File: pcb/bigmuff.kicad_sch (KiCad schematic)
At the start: 46 parts, among them Q1 BC549, Q2 BC549, Q3 BC549, Q4 BC549

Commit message: update pcb
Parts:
- C1, C6, C8: footprint Capacitor_THT:CP_Radial_Tantal_D4.5mm_P5.00mm -> Capacitor_THT:C_Axial_L5.1mm_D3.1mm_P7.50mm_Horizontal
- C10, C11, C12, C13, C2, C3, C4, C5, C7, C9: footprint Capacitor_THT:C_Disc_D4.3mm_W1.9mm_P5.00mm -> Capacitor_THT:C_Axial_L5.1mm_D3.1mm_P7.50mm_Horizontal
- R1, R10, R11, R12, R13, R14, R15, R16, R17, R18, R19, R2, R20, R21, R22, R3, R4, R5, R6, R7, R8, R9: footprint Resistor_THT:R_Axial_DIN0207_L6.3mm_D2.5mm_P7.62mm_Horizontal -> Resistor_THT:R_Axial_DIN0207_L6.3mm_D2.5mm_P10.16mm_Horizontal
- RV1, RV2, RV3: footprint Potentiometer_THT:Potentiometer_Alpha_RD901F-40-00D_Single_Vertical -> Potentiometer_THT:Potentiometer_Alps_RK09L_Single_Vertical
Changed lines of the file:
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@@
 			)
 		)
-		(property "Footprint" "Resistor_THT:R_Axial_DIN0207_L6.3mm_D2.5mm_P7.62mm_Horizontal"
+		(property "Footprint" "Resistor_THT:R_Axial_DIN0207_L6.3mm_D2.5mm_P10.16mm_Horizontal"
 			(at 34.29 66.802 90)
 			(effects
@@
 			)
 		)
-		(property "Footprint" "Resistor_THT:R_Axial_DIN0207_L6.3mm_D2.5mm_P7.62mm_Horizontal"
+		(property "Footprint" "Resistor_THT:R_Axial_DIN0207_L6.3mm_D2.5mm_P10.16mm_Horizontal"
 			(at 198.882 74.93 90)
 			(effects
@@
 			)
 		)
-		(property "Footprint" "Resistor_THT:R_Axial_DIN0207_L6.3mm_D2.5mm_P7.62mm_Horizontal"
+		(property "Footprint" "Resistor_THT:R_Axial_DIN0207_L6.3mm_D2.5mm_P10.16mm_Horizontal"
 			(at 53.34 165.608 90)
 			(effects
@@
 			)
 		)
-		(property "Footprint" "Resistor_THT:R_Axial_DIN0207_L6.3mm_D2.5mm_P7.62mm_Horizontal"
+		(property "Footprint" "Resistor_THT:R_Axial_DIN0207_L6.3mm_D2.5mm_P10.16mm_Horizontal"
 			(at 69.342 81.28 90)
 			(effects
@@
 			)
 		)
-		(property "Footprint" "Resistor_THT:R_Axial_DIN0207_L6.3mm_D2.5mm_P7.62mm_Horizontal"
+		(property "Footprint" "Resistor_THT:R_Axial_DIN0207_L6.3mm_D2.5mm_P10.16mm_Horizontal"
 			(at 198.882 49.53 90)
 			(effects
@@
 			)
 		)
-		(property "Footprint" "Resistor_THT:R_Axial_DIN0207_L6.3mm_D2.5mm_P7.62mm_Horizontal"
+		(property "Footprint" "Resistor_THT:R_Axial_DIN0207_L6.3mm_D2.5mm_P10.16mm_Horizontal"
 			(at 210.312 49.53 90)
 			(effects
@@
 			)
 		)
-		(property "Footprint" "Resistor_THT:R_Axial_DIN0207_L6.3mm_D2.5mm_P7.62mm_Horizontal"
+		(property "Footprint" "Resistor_THT:R_Axial_DIN0207_L6.3mm_D2.5mm_P10.16mm_Horizontal"
 			(at 73.66 157.988 90)
 			(effects
@@
 			)
 		)
-		(property "Footprint" "Potentiometer_THT:Potentiometer_Alpha_RD901F-40-00D_Single_Vertical"
+		(property "Footprint" "Potentiometer_THT:Potentiometer_Alps_RK09L_Single_Vertical"
 			(at 146.05 63.5 0)
 			(effects
@@
 			)
 		)
-		(property "Footprint" "Capacitor_THT:C_Disc_D4.3mm_W1.9mm_P5.00mm"
+		(property "Footprint" "Capacitor_THT:C_Axial_L5.1mm_D3.1mm_P7.50mm_Horizontal"
 			(at 82.55 57.4548 0)
 			(effects
@@
 			)
 		)
-		(property "Footprint" "Capacitor_THT:C_Disc_D4.3mm_W1.9mm_P5.00mm"
+		(property "Footprint" "Capacitor_THT:C_Axial_L5.1mm_D3.1mm_P7.50mm_Horizontal"
 			(at 66.04 44.7548 0)
 			(effects
@@
 			)
 		)
-		(property "Footprint" "Potentiometer_THT:Potentiometer_Alpha_RD901F-40-00D_Single_Vertical"
+		(property "Footprint" "Potentiometer_THT:Potentiometer_Alps_RK09L_Single_Vertical"
 			(at 85.09 68.58 0)
 			(effects
@@
 			)
 		)
-		(property "Footprint" "Capacitor_THT:C_Disc_D4.3mm_W1.9mm_P5.00mm"
+		(property "Footprint" "Capacitor_THT:C_Axial_L5.1mm_D3.1mm_P7.50mm_Horizontal"
 			(at 46.99 162.8648 0)
 			(effects
@@
 			)
 		)
-		(property "Footprint" "Potentiometer_THT:Potentiometer_Alpha_RD901F-40-00D_Single_Vertical"
+		(property "Footprint" "Potentiometer_THT:Potentiometer_Alps_RK09L_Single_Vertical"
 			(at 232.41 66.04 0)
 			(effects
@@
 			)
 		)
-		(property "Footprint" "Resistor_THT:R_Axial_DIN0207_L6.3mm_D2.5mm_P7.62mm_Horizontal"
+		(property "Footprint" "Resistor_THT:R_Axial_DIN0207_L6.3mm_D2.5mm_P10.16mm_Horizontal"
 			(at 113.792 173.99 90)
 			(effects
@@
 			)
 		)
-		(property "Footprint" "Resistor_THT:R_Axial_DIN0207_L6.3mm_D2.5mm_P7.62mm_Horizontal"
+		(property "Footprint" "Resistor_THT:R_Axial_DIN0207_L6.3mm_D2.5mm_P10.16mm_Horizontal"
 			(at 109.22 165.608 90)
 			(effects
@@
 			)
 		)
-		(property "Footprint" "Capacitor_THT:C_Disc_D4.3mm_W1.9mm_P5.00mm"
+		(property "Footprint" "Capacitor_THT:C_Axial_L5.1mm_D3.1mm_P7.50mm_Horizontal"
 			(at 195.58 59.9948 0)
 			(effects
@@
 			)
 		)
-		(property "Footprint" "Resistor_THT:R_Axial_DIN0207_L6.3mm_D2.5mm_P7.62mm_Horizontal"
+		(property "Footprint" "Resistor_THT:R_Axial_DIN0207_L6.3mm_D2.5mm_P10.16mm_Horizontal"
 			(at 144.272 46.99 90)
 			(effects
@@
 			)
 		)
-		(property "Footprint" "Capacitor_THT:CP_Radial_Tantal_D4.5mm_P5.00mm"
+		(property "Footprint" "Capacitor_THT:C_Axial_L5.1mm_D3.1mm_P7.50mm_Horizontal"
 			(at 62.23 129.2352 0)
 			(effects
@@
 			)
 		)
-		(property "Footprint" "Resistor_THT:R_Axial_DIN0207_L6.3mm_D2.5mm_P7.62mm_Horizontal"
+		(property "Footprint" "Resistor_THT:R_Axial_DIN0207_L6.3mm_D2.5mm_P10.16mm_Horizontal"
 			(at 128.27 157.988 90)
 			(effects
@@
 			)
 		)
-		(property "Footprint" "Capacitor_THT:C_Disc_D4.3mm_W1.9mm_P5.00mm"
+		(property "Footprint" "Capacitor_THT:C_Axial_L5.1mm_D3.1mm_P7.50mm_Horizontal"
 			(at 140.97 53.6448 0)
 			(effects
@@
 			)
 		)
-		(property "Footprint" "Resistor_THT:R_Axial_DIN0207_L6.3mm_D2.5mm_P7.62mm_Horizontal"
+		(property "Footprint" "Resistor_THT:R_Axial_DIN0207_L6.3mm_D2.5mm_P10.16mm_Horizontal"
 			(at 84.582 119.38 90)
 			(effects
@@
 			)
 		)
-		(property "Footprint" "Resistor_THT:R_Axial_DIN0207_L6.3mm_D2.5mm_P7.62mm_Horizontal"
+		(property "Footprint" "Resistor_THT:R_Axial_DIN0207_L6.3mm_D2.5mm_P10.16mm_Horizontal"
 			(at 50.292 81.28 90)
 			(effects
@@
 			)
 		)
-		(property "Footprint" "Resistor_THT:R_Axial_DIN0207_L6.3mm_D2.5mm_P7.62mm_Horizontal"
+		(property "Footprint" "Resistor_THT:R_Axial_DIN0207_L6.3mm_D2.5mm_P10.16mm_Horizontal"
 			(at 62.23 60.198 90)
 			(effects
@@
 			)
 		)
-		(property "Footprint" "Capacitor_THT:CP_Radial_Tantal_D4.5mm_P5.00mm"
+		(property "Footprint" "Capacitor_THT:C_Axial_L5.1mm_D3.1mm_P7.50mm_Horizontal"
 			(at 40.64 69.5452 0)
 			(effects
@@
 			)
 		)
-		(property "Footprint" "Resistor_THT:R_Axial_DIN0207_L6.3mm_D2.5mm_P7.62mm_Horizontal"
+		(property "Footprint" "Resistor_THT:R_Axial_DIN0207_L6.3mm_D2.5mm_P10.16mm_Horizontal"
 			(at 210.312 74.93 90)
 			(effects
@@
 			)
 		)
-		(property "Footprint" "Resistor_THT:R_Axial_DIN0207_L6.3mm_D2.5mm_P7.62mm_Horizontal"
+		(property "Footprint" "Resistor_THT:R_Axial_DIN0207_L6.3mm_D2.5mm_P10.16mm_Horizontal"
 			(at 83.312 81.28 90)
 			(effects
@@
 			)
 		)
-		(property "Footprint" "Capacitor_THT:CP_Radial_Tantal_D4.5mm_P5.00mm"
+		(property "Footprint" "Capacitor_THT:C_Axial_L5.1mm_D3.1mm_P7.50mm_Horizontal"
 			(at 116.84 130.5052 0)
 			(effects
@@
 			)
 		)
-		(property "Footprint" "Resistor_THT:R_Axial_DIN0207_L6.3mm_D2.5mm_P7.62mm_Horizontal"
+		(property "Footprint" "Resistor_THT:R_Axial_DIN0207_L6.3mm_D2.5mm_P10.16mm_Horizontal"
 			(at 139.192 173.99 90)
 			(effects
@@
 			)
 		)
-		(property "Footprint" "Capacitor_THT:C_Disc_D4.3mm_W1.9mm_P5.00mm"
+		(property "Footprint" "Capacitor_THT:C_Axial_L5.1mm_D3.1mm_P7.50mm_Horizontal"
 			(at 77.47 143.8148 0)
 			(effects
@@
 			)
 		)
-		(property "Footprint" "Resistor_THT:R_Axial_DIN0207_L6.3mm_D2.5mm_P7.62mm_Horizontal"
+		(property "Footprint" "Resistor_THT:R_Axial_DIN0207_L6.3mm_D2.5mm_P10.16mm_Horizontal"
 			(at 59.182 173.99 90)
 			(effects
@@
 			)
 		)
-		(property "Footprint" "Capacitor_THT:C_Disc_D4.3mm_W1.9mm_P5.00mm"
+		(property "Footprint" "Capacitor_THT:C_Axial_L5.1mm_D3.1mm_P7.50mm_Horizontal"
 			(at 145.0848 74.93 0)
 			(effects
@@
 			)
 		)
-		(property "Footprint" "Resistor_THT:R_Axial_DIN0207_L6.3mm_D2.5mm_P7.62mm_Horizontal"
+		(property "Footprint" "Resistor_THT:R_Axial_DIN0207_L6.3mm_D2.5mm_P10.16mm_Horizontal"
 			(at 84.582 173.99 90)
 			(effects
@@
 			)
 		)
-		(property "Footprint" "Resistor_THT:R_Axial_DIN0207_L6.3mm_D2.5mm_P7.62mm_Horizontal"
+		(property "Footprint" "Resistor_THT:R_Axial_DIN0207_L6.3mm_D2.5mm_P10.16mm_Horizontal"
 			(at 137.16 69.342 90)
 			(effects
@@
 			)
 		)
-		(property "Footprint" "Resistor_THT:R_Axial_DIN0207_L6.3mm_D2.5mm_P7.62mm_Horizontal"
+		(property "Footprint" "Resistor_THT:R_Axial_DIN0207_L6.3mm_D2.5mm_P10.16mm_Horizontal"
 			(at 139.192 119.38 90)
 			(effects
@@
 			)
 		)
-		(property "Footprint" "Capacitor_THT:C_Disc_D4.3mm_W1.9mm_P5.00mm"
+		(property "Footprint" "Capacitor_THT:C_Axial_L5.1mm_D3.1mm_P7.50mm_Horizontal"
 			(at 228.6 53.6448 0)
 			(effects
@@
 			)
 		)
-		(property "Footprint" "Capacitor_THT:C_Disc_D4.3mm_W1.9mm_P5.00mm"
+		(property "Footprint" "Capacitor_THT:C_Axial_L5.1mm_D3.1mm_P7.50mm_Horizontal"
 			(at 101.6 162.8648 0)
 			(effects
@@
 			)
 		)
-		(property "Footprint" "Resistor_THT:R_Axial_DIN0207_L6.3mm_D2.5mm_P7.62mm_Horizontal"
+		(property "Footprint" "Resistor_THT:R_Axial_DIN0207_L6.3mm_D2.5mm_P10.16mm_Horizontal"
 			(at 69.342 38.1 90)
 			(effects
@@
 			)
 		)
-		(property "Footprint" "Capacitor_THT:C_Disc_D4.3mm_W1.9mm_P5.00mm"
+		(property "Footprint" "Capacitor_THT:C_Axial_L5.1mm_D3.1mm_P7.50mm_Horizontal"
 			(at 132.08 143.8148 0)
 			(effects

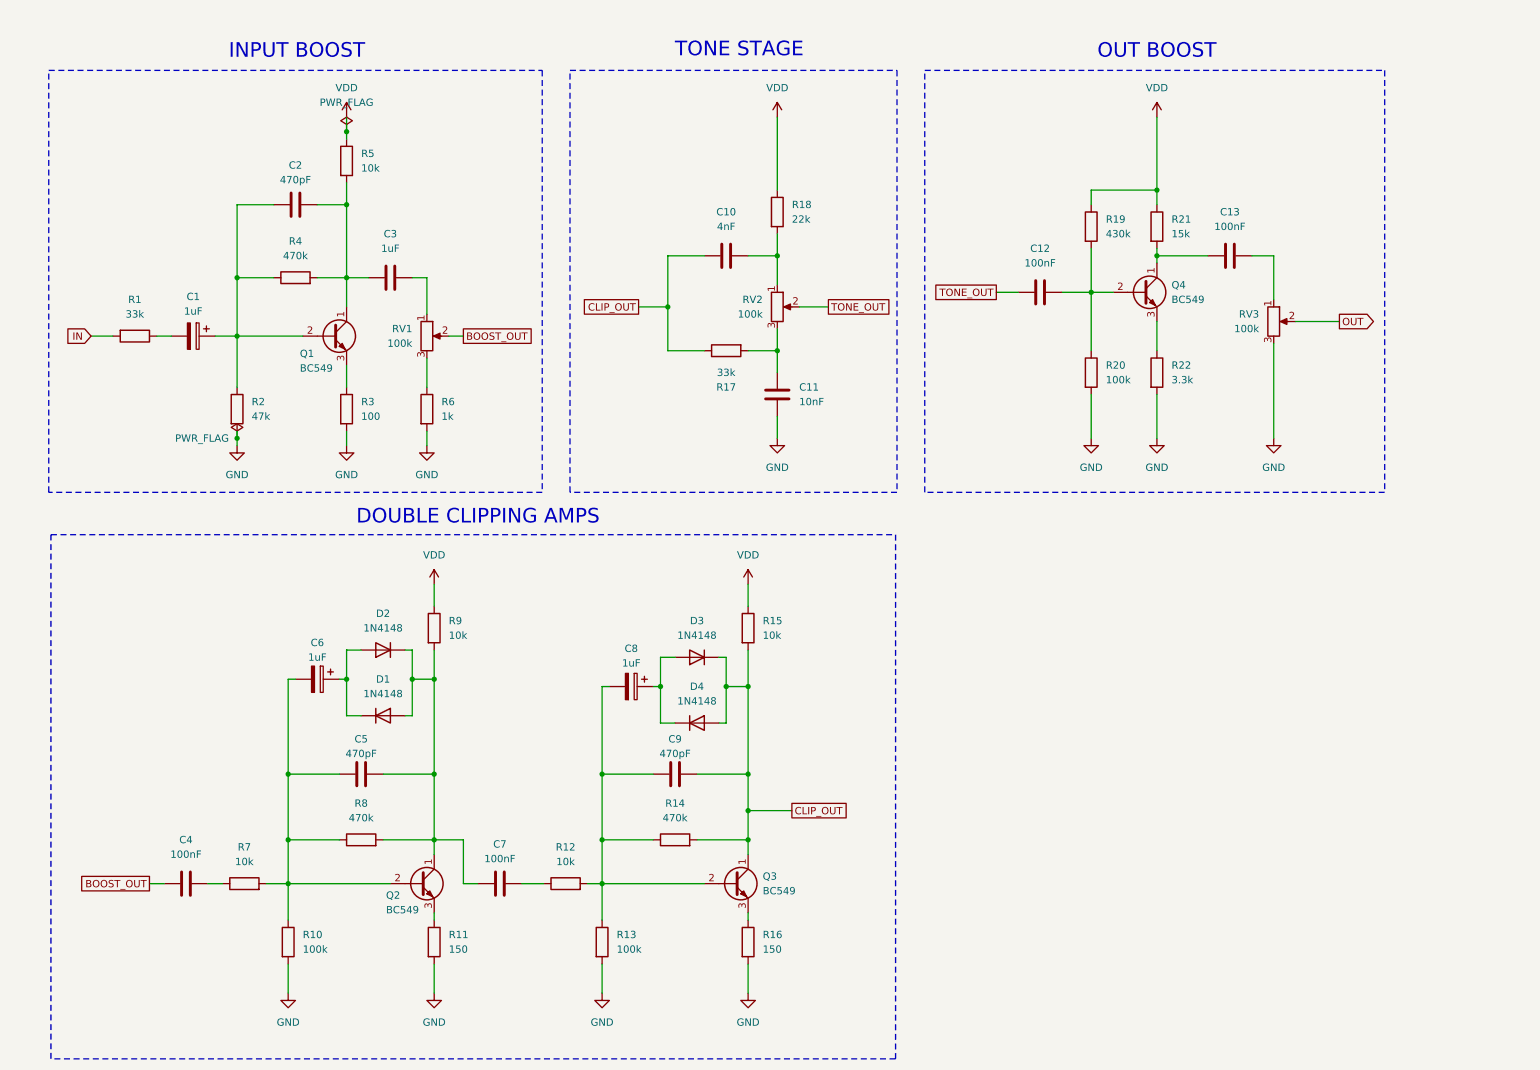
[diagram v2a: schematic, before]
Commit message: updated pcb
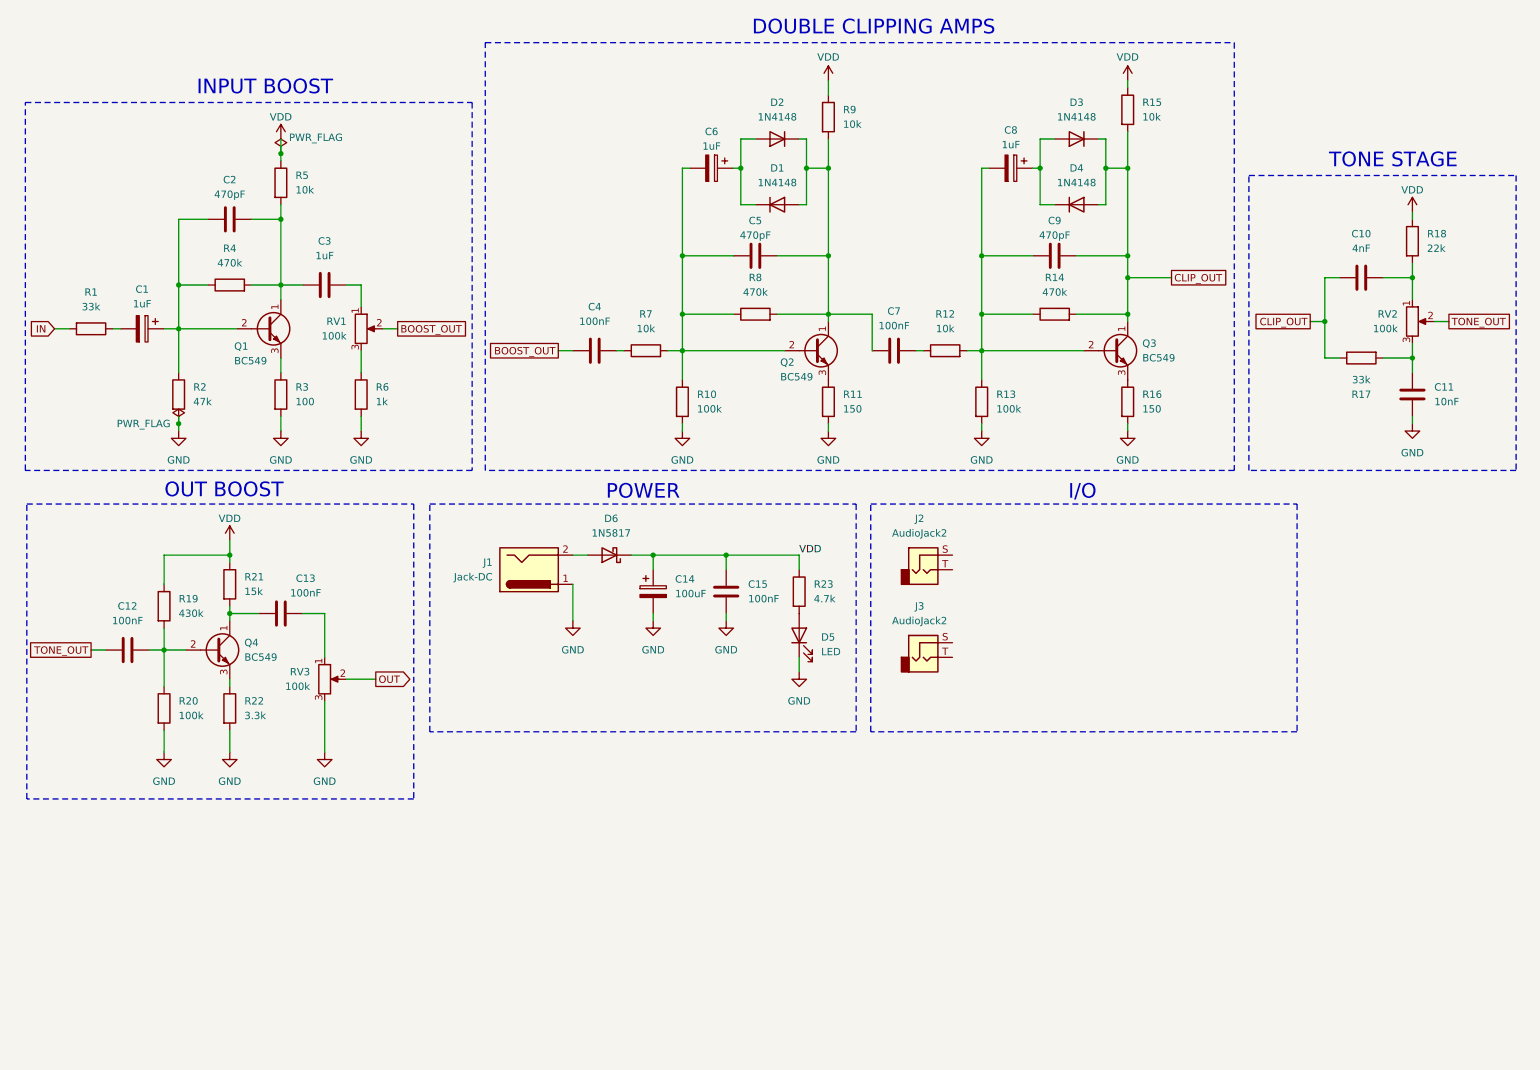
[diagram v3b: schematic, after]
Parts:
- added C14: 100uF, Capacitor_THT:CP_Radial_D6.3mm_P2.50mm, symbol Device:C_Polarized
- added C15: 100nF, Capacitor_THT:C_Axial_L5.1mm_D3.1mm_P7.50mm_Horizontal, symbol Device:C
- added D5: LED, LED_THT:LED_D5.0mm, symbol Device:LED
- added D6: 1N5817, Diode_THT:D_DO-41_SOD81_P10.16mm_Horizontal, symbol Diode:1N5817
- added J1: Jack-DC, Connector_BarrelJack:BarrelJack_Kycon_KLDX-0202-xC_Horizontal, symbol Connector:Jack-DC
- added J2, J3: AudioJack2, Connector_Audio:Jack_6.35mm_Neutrik_NRJ3HF-1_Horizontal, symbol Connector_Audio:AudioJack2
- added R23: 4.7k, Resistor_THT:R_Axial_DIN0207_L6.3mm_D2.5mm_P10.16mm_Horizontal, symbol Device:R
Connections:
- net GND: now also C14.2, C15.2, D5.1 (K), J1.1
- net VDD: now also C14.1, C15.1, D6.1 (K), R23.1
- new net: D5.2 (A), R23.2
- new net: D6.2 (A), J1.2
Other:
- note added: "I/O"
- note added: "POWER"
- moved on the sheet: C1, C10, C11, C12, C13, C2, C3, C4, C5, C6, C7, C8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
